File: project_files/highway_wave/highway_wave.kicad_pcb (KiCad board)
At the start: 2 copper layers, 10 parts, among them U1 GW1N-LV9QN88C6_I5_, U4 PAM8403D

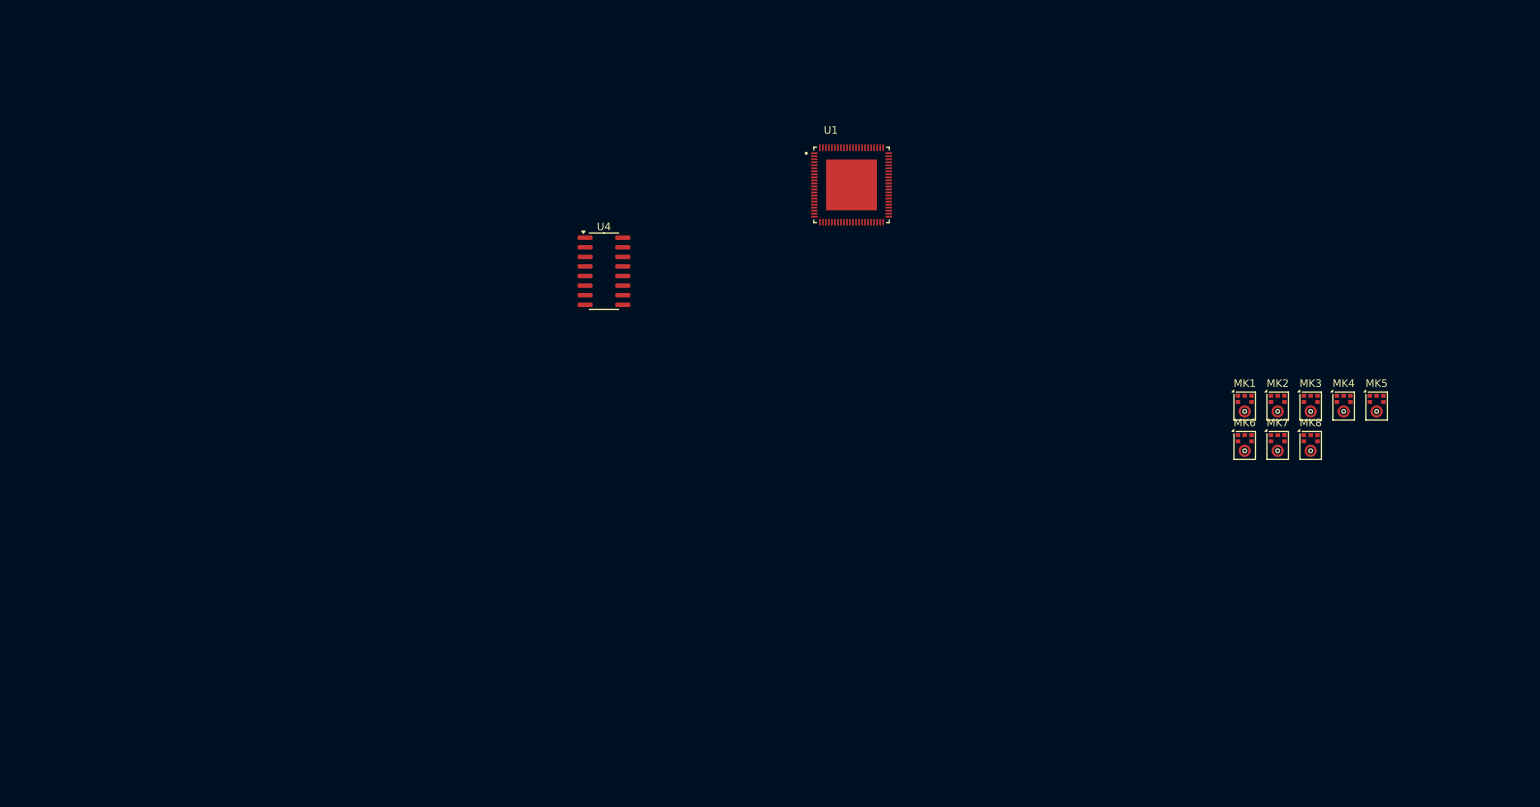
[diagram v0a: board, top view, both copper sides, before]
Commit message: random committ
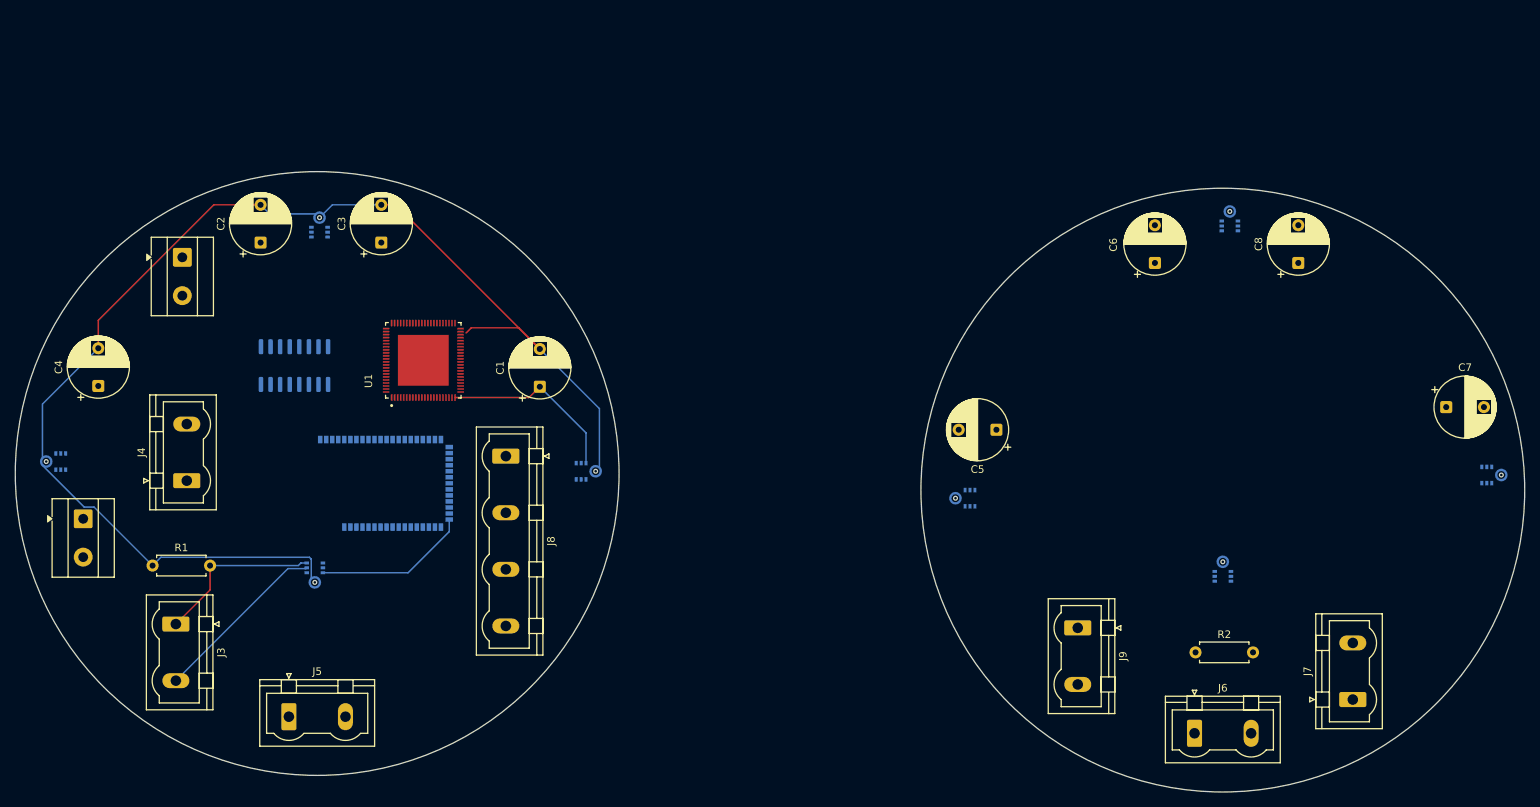
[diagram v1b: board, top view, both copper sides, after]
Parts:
- added C1: 1 uF, Capacitor_THT:CP_Radial_D8.0mm_P5.00mm, F.Cu at (116.5, 96.3)
- added C2: 1 uF, Capacitor_THT:CP_Radial_D8.0mm_P5.00mm, F.Cu at (79.5, 77.2)
- added C3: 1 uF, Capacitor_THT:CP_Radial_D8.0mm_P5.00mm, F.Cu at (95.5, 77.2)
- added C4: 1 uF, Capacitor_THT:CP_Radial_D8.0mm_P5.00mm, F.Cu at (58.0, 96.2)
- added C5: 1 uF, Capacitor_THT:CP_Radial_D8.0mm_P5.00mm, F.Cu at (177.0, 102.0)
- added C6: 1 uF, Capacitor_THT:CP_Radial_D8.0mm_P5.00mm, F.Cu at (198.0, 79.9)
- added C7: 1 uF, Capacitor_THT:CP_Radial_D8.0mm_P5.00mm, F.Cu at (236.6, 99.0)
- added C8: 1 uF, Capacitor_THT:CP_Radial_D8.0mm_P5.00mm, F.Cu at (217.0, 79.9)
- added J1: Screw_Terminal_01x02, TerminalBlock_MetzConnect:TerminalBlock_MetzConnect_Type101_RT01602HBWC_1x02_P5.08mm_Horizontal, F.Cu at (56.0, 113.8)
- added J2: Screw_Terminal_01x02, TerminalBlock_MetzConnect:TerminalBlock_MetzConnect_Type101_RT01602HBWC_1x02_P5.08mm_Horizontal, F.Cu at (69.1, 79.2)
- added J3: Conn_01x02_Socket, Connector_Phoenix_GMSTB:PhoenixContact_GMSTBVA_2,5_2-G_1x02_P7.50mm_Vertical, F.Cu at (68.3, 127.8)
- added J4: Conn_01x02_Socket, Connector_Phoenix_GMSTB:PhoenixContact_GMSTBVA_2,5_2-G_1x02_P7.50mm_Vertical, F.Cu at (69.7, 108.8)
- added J5: Conn_01x02_Pin, Connector_Phoenix_GMSTB:PhoenixContact_GMSTBVA_2,5_2-G_1x02_P7.50mm_Vertical, F.Cu at (83.2, 140.0)
- added J6: Conn_01x02_Pin, Connector_Phoenix_GMSTB:PhoenixContact_GMSTBVA_2,5_2-G_1x02_P7.50mm_Vertical, F.Cu at (203.2, 142.2)
- added J7: Conn_01x02_Pin, Connector_Phoenix_GMSTB:PhoenixContact_GMSTBVA_2,5_2-G_1x02_P7.50mm_Vertical, F.Cu at (224.2, 137.8)
- added J8: Conn_01x04_Socket, Connector_Phoenix_GMSTB:PhoenixContact_GMSTBVA_2,5_4-G_1x04_P7.50mm_Vertical, F.Cu at (112.0, 105.5)
- added J9: Conn_01x02_Pin, Connector_Phoenix_GMSTB:PhoenixContact_GMSTBVA_2,5_2-G_1x02_P7.50mm_Vertical, F.Cu at (187.8, 128.2)
- added R1: 100 k, Resistor_THT:R_Axial_DIN0207_L6.3mm_D2.5mm_P7.62mm_Horizontal, F.Cu at (65.2, 120.0)
- added R2: 100 k, Resistor_THT:R_Axial_DIN0207_L6.3mm_D2.5mm_P7.62mm_Horizontal, F.Cu at (203.4, 131.5)
- added U2: MOUDLE-BLUETOOTH-AUDIO-BC127_51P-18X11.8MM_, MOUDLE-BLUETOOTH-AUDIO-BC127_51P-18X11.8MM_:LGA51-0.8-18X11.8MM, B.Cu at (95.5, 109.1)
- MK1, MK2, MK3, MK4, MK5, MK6, MK7, MK8: value ICS-43434 -> ICS-52000; footprint Sensor_Audio:InvenSense_ICS-43434-6_3.5x2.65mm -> wave:MIC_ICS-52000; moved to B.Cu
- U4: moved to B.Cu
- moved MK4 171.2 mm to (52.0, 106.2), turned to 90 degrees
- moved MK3 133.9 mm to (86.7, 121.3), turned to 180 degrees
- moved MK2 129.2 mm to (87.3, 74.8)
- moved MK1 87.3 mm to (123.0, 107.5), turned to -90 degrees
- moved U1 61.3 mm to (101.1, 92.8), turned to 90 degrees
- moved MK5 56.2 mm to (172.5, 111.1), turned to 90 degrees
- moved U4 42.9 mm to (84.0, 93.5), turned to -90 degrees
- moved MK6 30.2 mm to (207.9, 74.0)
- moved MK7 29.0 mm to (243.0, 108.0), turned to -90 degrees
- moved MK8 20.0 mm to (207.0, 120.4)
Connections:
- MK1 pad 1: Net-(MK1-WS) -> WSO Mk1
- MK1 pad 2: GND -> +3V3
- MK1 pad 3: GND -> +3V3
- MK1 pad 5: VCC -> Net-(J5-Pin_2)
- MK1 pad 6: Net-(MK1-SD) -> TDM CLK
- MK2 pad 1: Net-(MK1-WS) -> WSO Mk2
- MK2 pad 2: GND -> +3V3
- MK2 pad 3: GND -> +3V3
- MK2 pad 5: VCC -> WSO Mk1
- MK2 pad 6: Net-(MK1-SD) -> TDM CLK
- MK3 pad 1: Net-(MK1-WS) -> WSO Mk3
- MK3 pad 2: GND -> +3V3
- MK3 pad 3: GND -> +3V3
- MK3 pad 5: VCC -> WSO Mk2
- MK3 pad 6: Net-(MK1-SD) -> TDM CLK
- MK4 pad 1: Net-(MK1-WS) -> Net-(J5-Pin_1)
- MK4 pad 2: GND -> +3V3
- MK4 pad 3: GND -> +3V3
- MK4 pad 5: VCC -> WSO Mk3
- MK4 pad 6: Net-(MK1-SD) -> TDM CLK
- MK5 pad 1: Net-(MK1-WS) -> WSO Mk5
- MK5 pad 2: VCC -> Net-(J7-Pin_1)
- MK5 pad 3: GND -> Net-(J7-Pin_1)
- MK5 pad 5: VCC -> Net-(J9-Pin_1)
- MK5 pad 6: Net-(MK1-SD) -> Net-(J6-Pin_2)
- MK6 pad 1: Net-(MK1-WS) -> WSO Mk6
- MK6 pad 2: VCC -> Net-(J7-Pin_1)
- MK6 pad 3: GND -> Net-(J7-Pin_1)
- MK6 pad 5: VCC -> WSO Mk5
- MK6 pad 6: Net-(MK1-SD) -> Net-(J6-Pin_2)
- MK7 pad 1: Net-(MK1-WS) -> unconnected-(MK7-WSO-Pad1)
- MK7 pad 2: VCC -> Net-(J7-Pin_1)
- MK7 pad 3: GND -> Net-(J7-Pin_1)
- MK7 pad 5: VCC -> unconnected-(MK7-WS-Pad5)
- MK7 pad 6: Net-(MK1-SD) -> Net-(J6-Pin_2)
- MK8 pad 1: Net-(MK1-WS) -> unconnected-(MK8-WSO-Pad1)
- MK8 pad 2: VCC -> Net-(J7-Pin_1)
- MK8 pad 3: GND -> Net-(J7-Pin_1)
- MK8 pad 5: VCC -> unconnected-(MK8-WS-Pad5)
- MK8 pad 6: Net-(MK1-SD) -> Net-(J6-Pin_2)
- U1 pad 1: Net-(U1-VCC-Pad1) -> +3V3
- U1 pad 11: unconnected-(U1-IOL15A/GCLKT_6-Pad11) -> Net-(U1-IOL15A/GCLKT_6)
- U1 pad 15: unconnected-(U1-IOL26A-Pad15) -> Net-(U1-IOL26A)
- U1 pad 2: Net-(U1-VSS-Pad2) -> GND
- U1 pad 21: Net-(U1-VSS-Pad2) -> GND
- U1 pad 22: Net-(U1-VCC-Pad1) -> +3V3
- U1 pad 24: Net-(U1-VSS-Pad2) -> GND
- U1 pad 27: unconnected-(U1-IOB11A-Pad27) -> Net-(U1-IOB11A)
- U1 pad 29: unconnected-(U1-IOB13A-Pad29) -> Net-(U1-IOB13A)
- U1 pad 43: Net-(U1-VSS-Pad2) -> GND
- U1 pad 45: Net-(U1-VCC-Pad1) -> +3V3
- U1 pad 46: Net-(U1-VSS-Pad2) -> GND
- U1 pad 52: unconnected-(U1-IOR17A/GCLKT_3-Pad52) -> TDM CLK
- U1 pad 65: Net-(U1-VSS-Pad2) -> GND
- U1 pad 66: Net-(U1-VCC-Pad1) -> +3V3
- U1 pad 80: unconnected-(U1-IOT12A-Pad80) -> TDM WS
- U1 pad 82: unconnected-(U1-IOT11A-Pad82) -> TDM SD
- U4 pad 10: unconnected-(U4-INR-Pad10) -> Net-(U1-IOB13A)
- U4 pad 7: unconnected-(U4-INL-Pad7) -> Net-(U1-IOB11A)
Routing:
- net GND: track 0.00 -> 168.5 mm
- net +3V3: track 0.00 -> 45.1 mm
- net TDM CLK: track 0.00 -> 23.5 mm
- net TDM SD: track 0.00 -> 22.6 mm
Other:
- board outline added: 200 x 82.2 mm

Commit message: fixed pcb
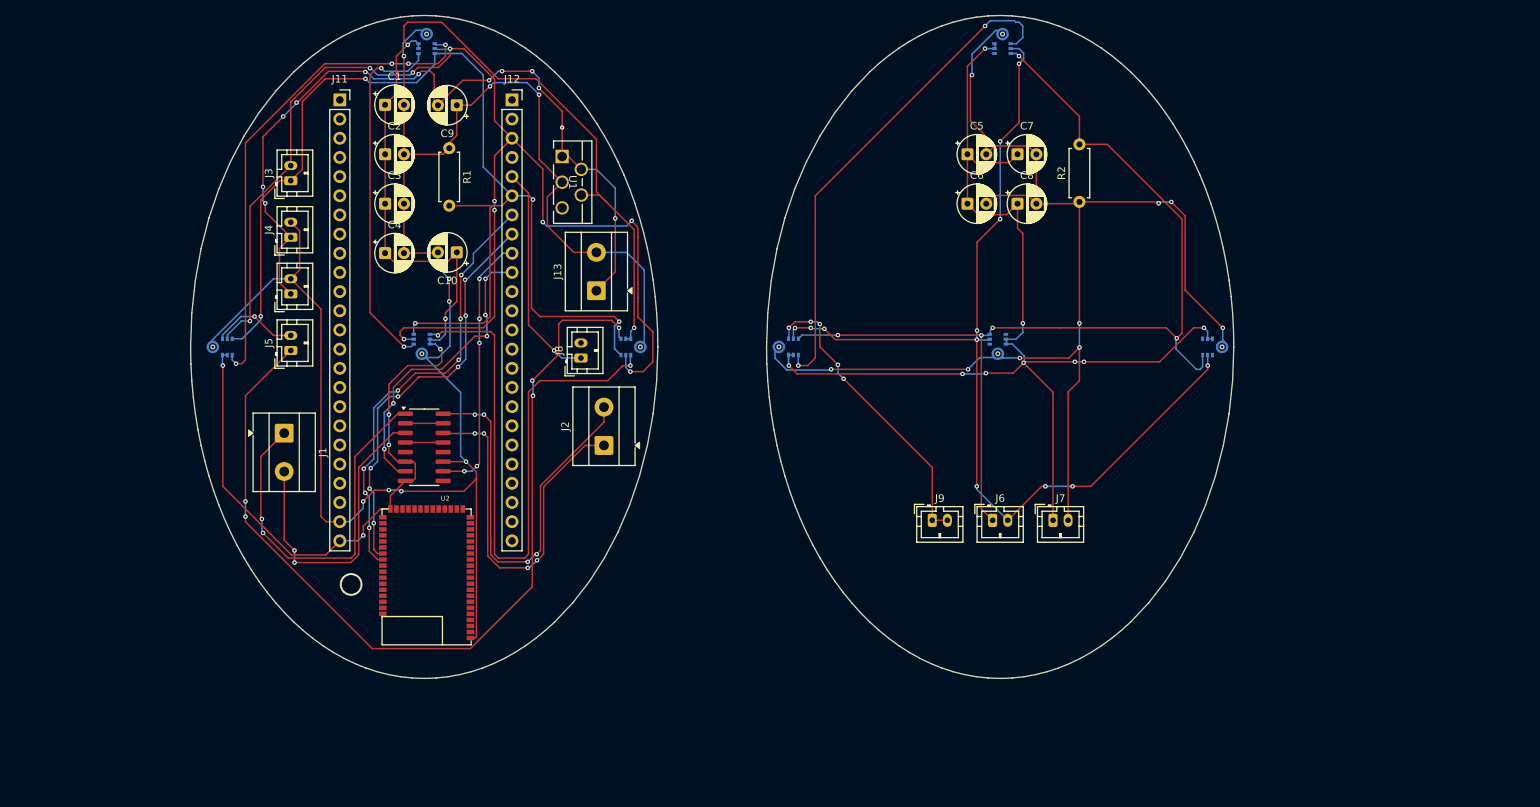
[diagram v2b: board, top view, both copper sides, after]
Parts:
- added C10: 47 uF, Capacitor_THT:CP_Radial_D5.0mm_P2.50mm, F.Cu at (105.5, 78.5)
- added C9: 1 uF, Capacitor_THT:CP_Radial_D5.0mm_P2.50mm, F.Cu at (105.5, 59.0)
- added J10: Conn_01x02_Socket, Connector_JST:JST_PH_B2B-PH-K_1x02_P2.00mm_Vertical, F.Cu at (83.5, 84.0)
- added J11: Conn_01x24, Connector_PinSocket_2.54mm:PinSocket_1x24_P2.54mm_Vertical, F.Cu at (90.0, 58.3)
- added J12: Conn_01x24, Connector_PinSocket_2.54mm:PinSocket_1x24_P2.54mm_Vertical, F.Cu at (112.8, 58.3)
- added J13: Screw_Terminal_01x02, TerminalBlock_MetzConnect:TerminalBlock_MetzConnect_Type101_RT01602HBWC_1x02_P5.08mm_Horizontal, F.Cu at (124.0, 83.6)
- C1, C2, C3, C4, C5, C6, C7, C8: footprint Capacitor_THT:CP_Radial_D8.0mm_P5.00mm -> Capacitor_THT:CP_Radial_D5.0mm_P2.50mm
- J3, J4, J5, J6, J7, J9: footprint Connector_Phoenix_GMSTB:PhoenixContact_GMSTBVA_2,5_2-G_1x02_P7.50mm_Vertical -> Connector_JST:JST_PH_B2B-PH-K_1x02_P2.00mm_Vertical
- J8: footprint Connector_Phoenix_GMSTB:PhoenixContact_GMSTBVA_2,5_4-G_1x04_P7.50mm_Vertical -> Connector_JST:JST_PH_B2B-PH-K_1x02_P2.00mm_Vertical
- U1: value GW1N-LV9QN88C6_I5_ -> TPS75633KC; footprint GW1N-LV9QN88C6_I5_:QFN40P1000X1000X95-89N -> footprints:KC5
- U2, U4: moved to F.Cu
- moved MK4 78.4 mm to (128.9, 91.0), turned to -90 degrees
- moved MK7 68.0 mm to (177.2, 91.0), turned to 180 degrees
- moved R1 67.9 mm to (104.5, 64.7), turned to -90 degrees
- moved C7 65.9 mm to (179.8, 65.5)
- moved R2 61.6 mm to (188.0, 71.8), turned to 90 degrees
- moved J2 61.2 mm to (125.0, 104.1), turned to 90 degrees
- moved J3 60.7 mm to (83.5, 69.0), turned to 90 degrees
- moved MK1 51.6 mm to (74.1, 91.0), turned to 90 degrees
- moved J5 48.5 mm to (83.5, 91.5), turned to 90 degrees
- moved J7 46.3 mm to (184.5, 114.0), turned to 0 degrees
- moved C1 42.6 mm to (96.0, 59.0), turned to 0 degrees
- moved C4 41.9 mm to (96.0, 78.6), turned to 0 degrees
- moved J6 38.9 mm to (176.5, 114.0)
- moved MK6 38.2 mm to (177.8, 50.5)
- moved C8 38.0 mm to (179.8, 72.0), turned to 0 degrees
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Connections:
- C1 pad 1: +3V3 -> Vout from Bat reg
- C1 pad 2: GND -> IN_GND
- C2 pad 1: +3V3 -> Vout from Bat reg
- C2 pad 2: GND -> IN_GND
- C3 pad 1: +3V3 -> Vout from Bat reg
- C3 pad 2: GND -> IN_GND
- C4 pad 1: +3V3 -> Vout from Bat reg
- C4 pad 2: GND -> IN_GND
- J3 pad 1: TDM SD -> 26_IOB8B
- J3 pad 2: TDM CLK -> 36_IOB29B
- J4 pad 1: +3V3 -> IN_3V3
- J4 pad 2: GND -> IN_GND
- J8 pad 1: TDM WS -> 25_IOB8A
- MK1 pad 2: +3V3 -> Vout from Bat reg
- MK1 pad 3: +3V3 -> Vout from Bat reg
- MK1 pad 4_1: GND -> IN_GND
- MK1 pad 4_2: GND -> IN_GND
- MK1 pad 4_3: GND -> IN_GND
- MK1 pad 4_4: GND -> IN_GND
- MK1 pad 6: TDM CLK -> 36_IOB29B
- MK1 pad 7: TDM SD -> 26_IOB8B
- MK2 pad 2: +3V3 -> Vout from Bat reg
- MK2 pad 3: +3V3 -> Vout from Bat reg
- MK2 pad 4_1: GND -> IN_GND
- MK2 pad 4_2: GND -> IN_GND
- MK2 pad 4_3: GND -> IN_GND
- MK2 pad 4_4: GND -> IN_GND
- MK2 pad 6: TDM CLK -> 36_IOB29B
- MK2 pad 7: TDM SD -> 26_IOB8B
- MK3 pad 2: +3V3 -> Vout from Bat reg
- MK3 pad 3: +3V3 -> Vout from Bat reg
- MK3 pad 4_1: GND -> IN_GND
- MK3 pad 4_2: GND -> IN_GND
- MK3 pad 4_3: GND -> IN_GND
- MK3 pad 4_4: GND -> IN_GND
- MK3 pad 6: TDM CLK -> 36_IOB29B
- MK3 pad 7: TDM SD -> 26_IOB8B
- MK4 pad 2: +3V3 -> Vout from Bat reg
- MK4 pad 3: +3V3 -> Vout from Bat reg
- MK4 pad 4_1: GND -> IN_GND
- MK4 pad 4_2: GND -> IN_GND
- MK4 pad 4_3: GND -> IN_GND
- MK4 pad 4_4: GND -> IN_GND
- MK4 pad 6: TDM CLK -> 36_IOB29B
- MK4 pad 7: TDM SD -> 26_IOB8B
- R1 pad 1: GND -> IN_GND
- R1 pad 2: TDM SD -> 26_IOB8B
- U1 pad 1: +3V3 -> IN_3V3
- U1 pad 2: GND -> IN_3V3
- U1 pad 3: unconnected-(U1-IOL2A-Pad3) -> IN_GND
- U1 pad 4: unconnected-(U1-IOL5A/JTAGSEL_N/LPLL_T_IN-Pad4) -> Vout from Bat reg
- U2 pad 1: GND -> IN_GND
- U2 pad 34: +3V3 -> Vout from Bat reg
- U2 pad 41: Net-(U1-IOL26A) -> 28_IOB11B
- U2 pad 42: Net-(U1-IOL15A/GCLKT_6) -> 27_IOB11A
- U4 pad 10: Net-(U1-IOB13A) -> 29_IOB13A
- U4 pad 11: GND -> IN_GND
- U4 pad 6: VCC -> Vout from Bat reg
- U4 pad 7: Net-(U1-IOB11A) -> 30_IOB13B
- U4 pad 8: VCC -> Vout from Bat reg
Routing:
- net IN_GND: track 0.00 -> 245.9 mm, vias 0 -> 9
- net Vout from Bat reg: track 0.00 -> 204.5 mm, vias 0 -> 8
- net 36_IOB29B: track 0.00 -> 170.7 mm, vias 0 -> 10
- net GND: track 168.5 -> 0.00 mm
- net Net-(J7-Pin_2): track 0.00 -> 165.7 mm, vias 0 -> 9
- net 26_IOB8B: track 0.00 -> 153.9 mm, vias 0 -> 5
- net Net-(J7-Pin_1): track 0.00 -> 148.4 mm, vias 0 -> 9
- net Net-(J6-Pin_1): track 0.00 -> 134.5 mm, vias 0 -> 5
- net Net-(J6-Pin_2): track 0.00 -> 133.0 mm, vias 0 -> 12
- net Net-(J5-Pin_1): track 0.00 -> 120.1 mm, vias 0 -> 5
- net IN_3V3: track 0.00 -> 105.8 mm, vias 0 -> 11
- net WSO Mk3: track 0.00 -> 80.8 mm, vias 0 -> 2
- net WSO Mk5: track 0.00 -> 66.3 mm, vias 0 -> 2
- net WSO Mk1: track 0.00 -> 65.8 mm, vias 0 -> 4
- net 27_IOB11A: track 0.00 -> 58.1 mm, vias 0 -> 7
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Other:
- board size 200 x 82.2 mm -> 138.2 x 87.8 mm
